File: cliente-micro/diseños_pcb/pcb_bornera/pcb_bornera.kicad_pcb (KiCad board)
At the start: 2 copper layers, 26.7 x 52.1 mm, 10 parts, among them J1 AC IN, J2 Bomba, J3 Pad-AC-Fuente-L, J4 Pad-AC-Fuente-N, J5 Pad-Relay-Comun, J6 Pad-Relay-NC

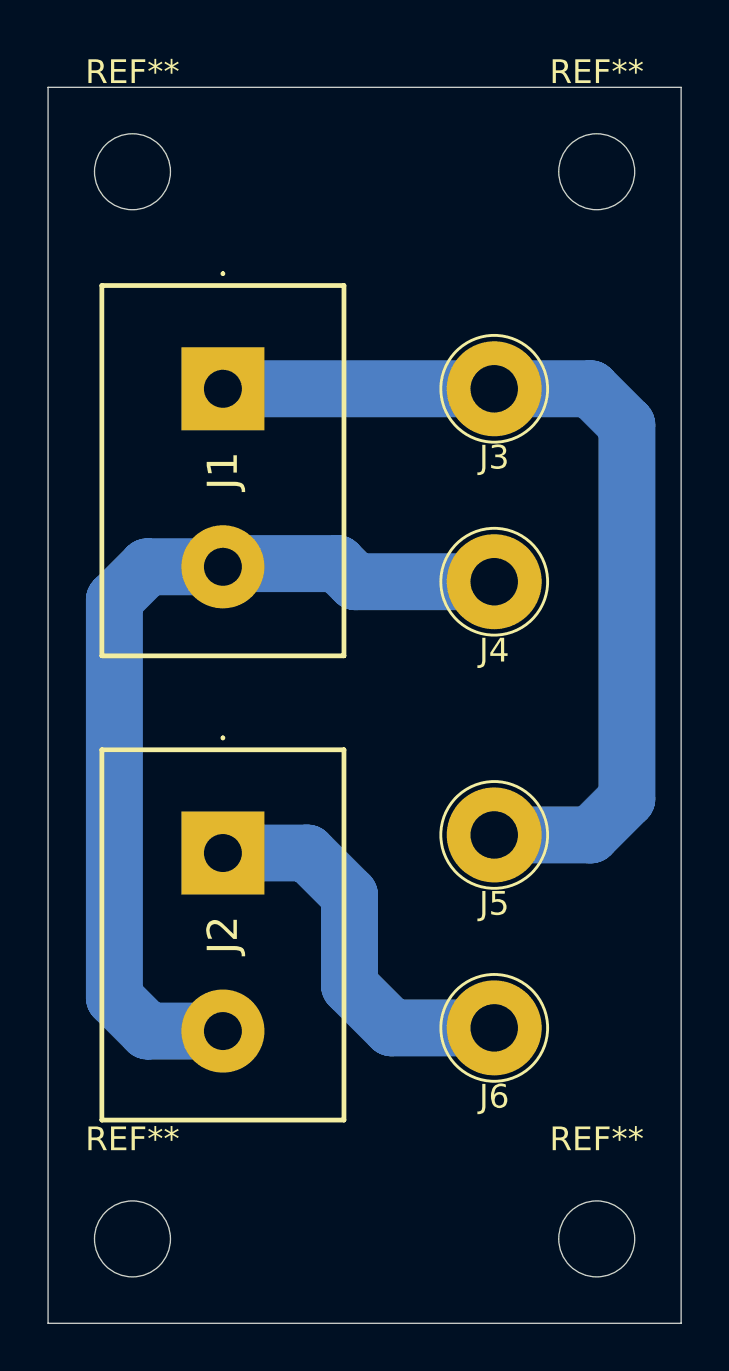
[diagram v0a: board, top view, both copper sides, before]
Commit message: Plot PCB
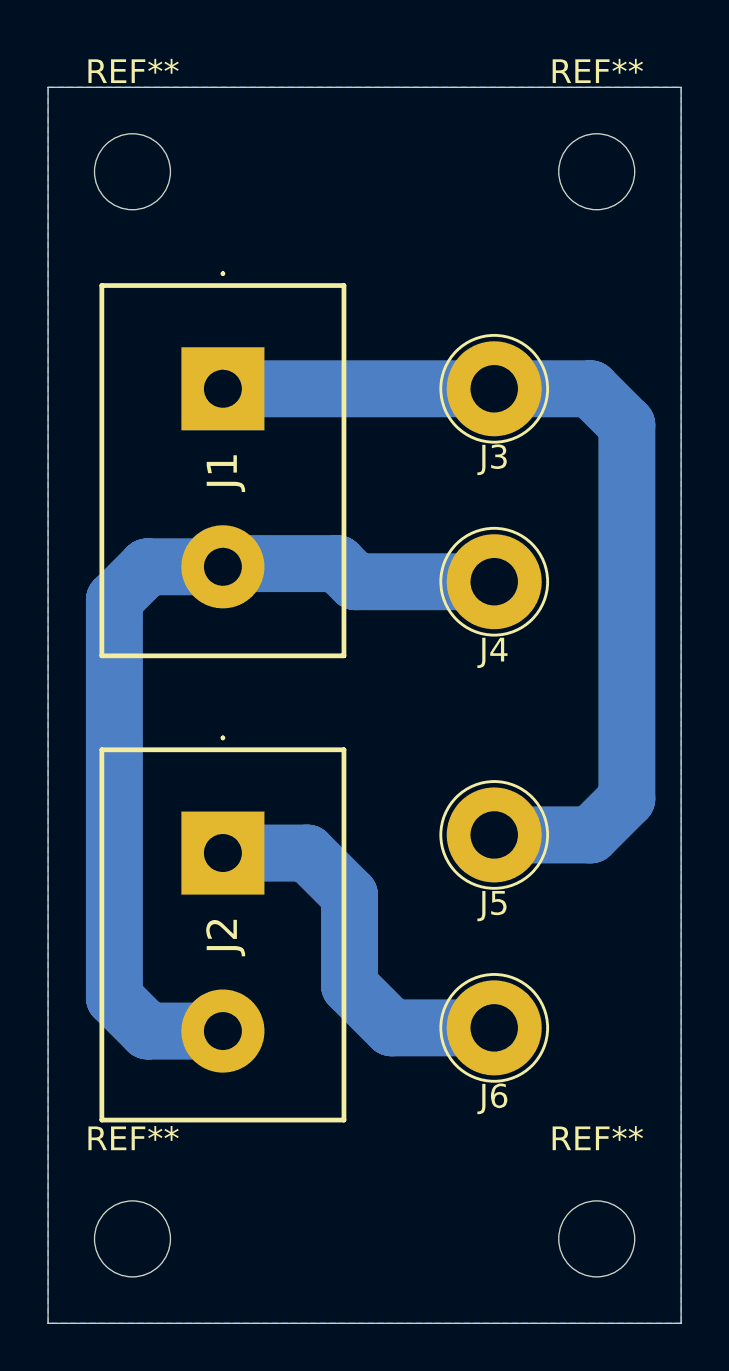
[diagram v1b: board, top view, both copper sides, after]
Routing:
- added copper zone on B.Cu, net (none)
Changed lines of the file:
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@@
 		(tenting front back)
 		(pcbplotparams
-			(layerselection 0x00000000_00000000_55555555_5755f5ff)
-			(plot_on_all_layers_selection 0x00000000_00000000_00000000_00000000)
+			(layerselection 0x00000000_00000000_55555555_55555554)
+			(plot_on_all_layers_selection 0x00000000_00000000_00000000_02020000)
 			(disableapertmacros no)
 			(usegerberextensions no)
@@
 			(hpglpenspeed 20)
 			(hpglpendiameter 15.000000)
-			(pdf_front_fp_property_popups yes)
-			(pdf_back_fp_property_popups yes)
-			(pdf_metadata yes)
+			(pdf_front_fp_property_popups no)
+			(pdf_back_fp_property_popups no)
+			(pdf_metadata no)
 			(pdf_single_document no)
 			(dxfpolygonmode yes)
@@
 			(psa4output no)
 			(plot_black_and_white yes)
-			(plotinvisibletext no)
 			(sketchpadsonfab no)
 			(plotpadnumbers no)
@@
 			(crossoutdnponfab yes)
 			(subtractmaskfromsilk no)
-			(outputformat 1)
-			(mirror no)
-			(drillshape 1)
+			(outputformat 4)
+			(mirror yes)
+			(drillshape 0)
 			(scaleselection 1)
 			(outputdirectory "")
@@
 			(fill no)
 			(layer "Cmts.User")
-			(net 256)
 		)
 		(fp_circle
@@
 			(fill no)
 			(layer "F.CrtYd")
-			(net 256)
 		)
 		(fp_text user "${REFERENCE}"
@@
 			(fill no)
 			(layer "Cmts.User")
-			(net 256)
 		)
 		(fp_circle
@@
 			(fill no)
 			(layer "F.CrtYd")
-			(net 256)
 		)
 		(fp_text user "${REFERENCE}"
@@
 	)
 	(gr_rect
+		(start 74.676 32.512)
+		(end 101.854 85.217)
+		(stroke
+			(width 0.1)
+			(type default)
+		)
+		(fill no)
+		(layer "Dwgs.User")
+	)
+	(gr_rect
 		(start 74.93 32.766)
 		(end 101.6 84.836)
@@
 		(layer "Edge.Cuts")
 	)
-	(dimension
-		(type orthogonal)
-		(layer "Dwgs.User")
-		(pts
-			(xy 93.726 64.262) (xy 93.726 72.39)
-		)
-		(height -6.096)
-		(orientation 1)
-		(format
-			(prefix "")
-			(suffix "")
-			(units 3)
-			(units_format 0)
-			(precision 4)
-			(suppress_zeroes yes)
-		)
-		(style
-			(thickness 0.1)
-			(arrow_length 1.27)
-			(text_position_mode 0)
-			(arrow_direction outward)
-			(extension_height 0.58642)
-			(extension_offset 0.5)
-			(keep_text_aligned yes)
-		)
-		(gr_text "8.128"
-			(at 86.48 68.326 90)
-			(layer "Dwgs.User")
-			(effects
-				(font
-					(size 1 1)
-					(thickness 0.15)
-				)
-			)
-		)
-	)
-	(dimension
-		(type orthogonal)
-		(layer "Dwgs.User")
-		(pts
-			(xy 93.726 53.594) (xy 93.726 45.466)
-		)
-		(height -3.81)
-		(orientation 1)
-		(format
-			(prefix "")
-			(suffix "")
-			(units 3)
-			(units_format 0)
-			(precision 4)
-			(suppress_zeroes yes)
-		)
-		(style
-			(thickness 0.1)
-			(arrow_length 1.27)
-			(text_position_mode 0)
-			(arrow_direction outward)
-			(extension_height 0.58642)
-			(extension_offset 0.5)
-			(keep_text_aligned yes)
-		)
-		(gr_text "8.128"
-			(at 88.766 49.53 90)
-			(layer "Dwgs.User")
-			(effects
-				(font
-					(size 1 1)
-					(thickness 0.15)
-				)
-			)
-		)
-	)
 	(segment
 		(start 99.314 62.738)
@@
 		(net 3)
 	)
+	(zone
+		(net 0)
+		(net_name "")
+		(layer "B.Cu")
+		(hatch edge 0.5)
+		(connect_pads
+			(clearance 1.524)
+		)
+		(min_thickness 0.25)
+		(filled_areas_thickness no)
+		(fill yes
+			(thermal_gap 0.5)
+			(thermal_bridge_width 0.5)
+			(island_removal_mode 1)
+			(island_area_min 9.999999)
+		)
+		(polygon
+			(pts
+				(xy 74.93 32.766) (xy 101.6 32.766) (xy 101.6 84.836) (xy 74.93 84.836)
+			)
+		)
+	)
 	(group ""
 		(members "244bb8b8-fbb5-482a-bc3a-28a81d2cf048" "a45ebb1b-2ab9-4f5e-b39f-677004642922")
@@
 		(members "b73f4011-b0a5-4c87-9d32-a3f4102b25b9" "ba66cba5-afbb-41a8-969f-94fd65750d74")
 	)
-	(group ""
-		(members "68f8fec0-0903-4d9b-8ad0-270cd186e6e3" "8d844b3f-0e39-4683-ac6b-72657b7ae727")
-	)
-	(group ""
-		(members "038f9dea-0b96-448d-8535-0cf601e2283e" "350ed1a8-0db7-4767-9416-b70ba5a73b6f")
-	)
 	(embedded_fonts no)
